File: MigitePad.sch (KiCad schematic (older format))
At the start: 74 parts, among them J1 OLED, J2 LED-Lily58-cache, SW1 SW_Push, SW2 Rotary_Encoder_Switch, U1 ProMicro

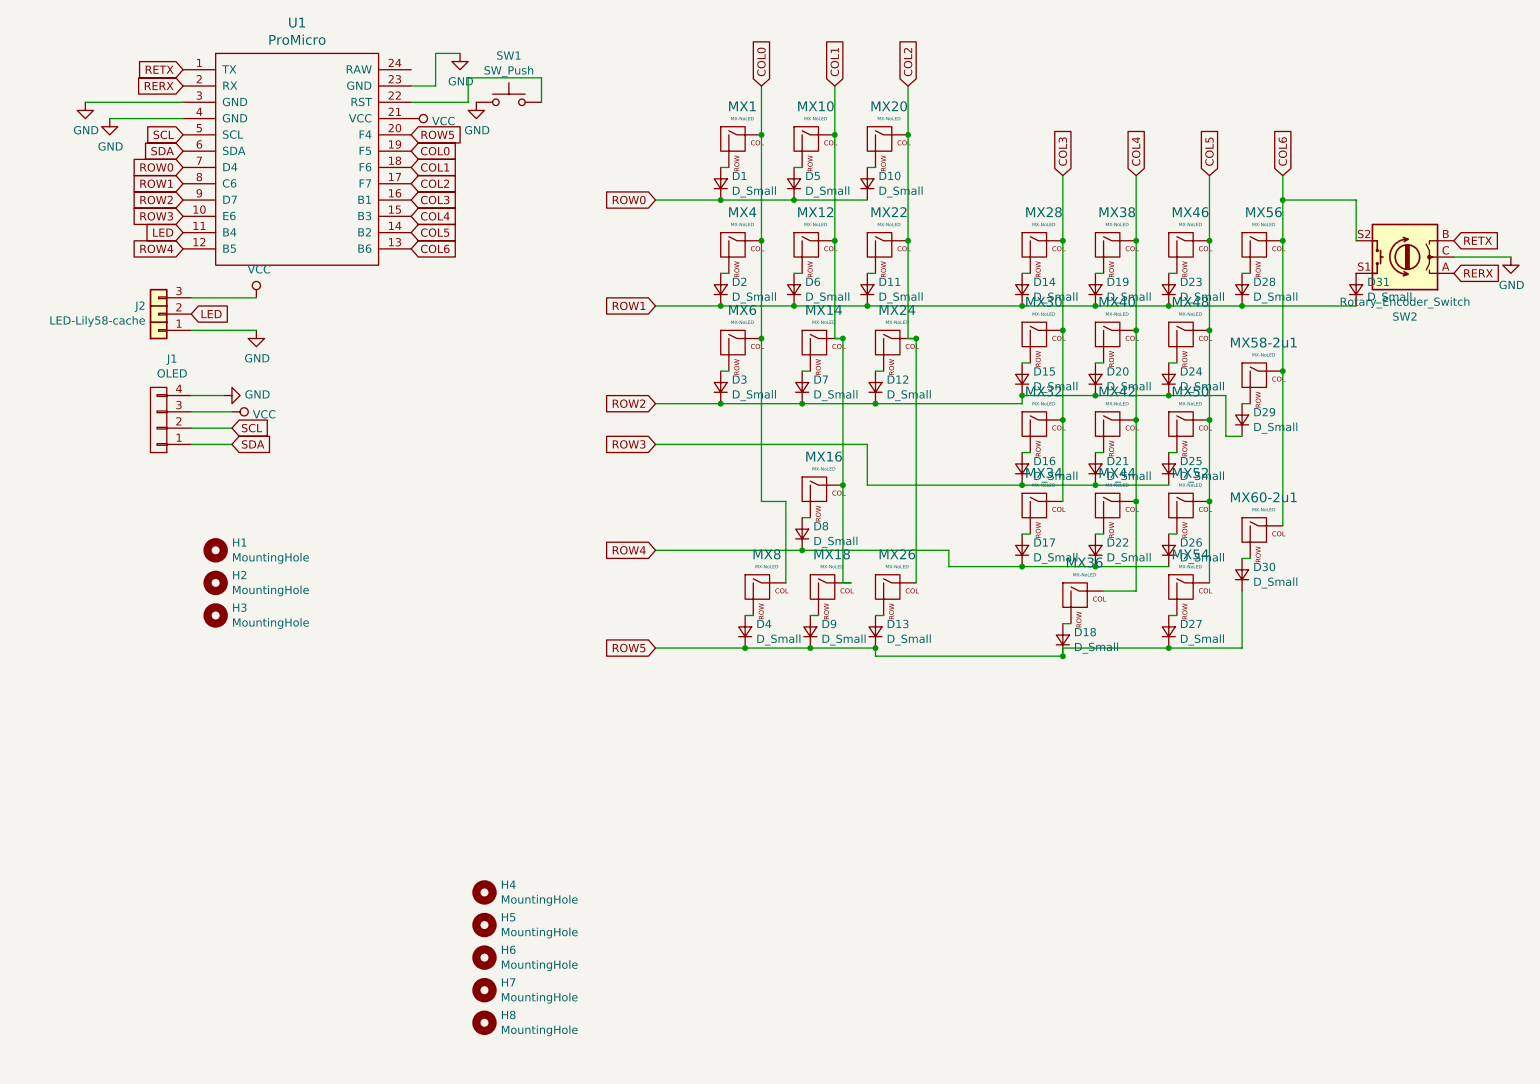
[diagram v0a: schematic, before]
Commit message: Rewired Encoder
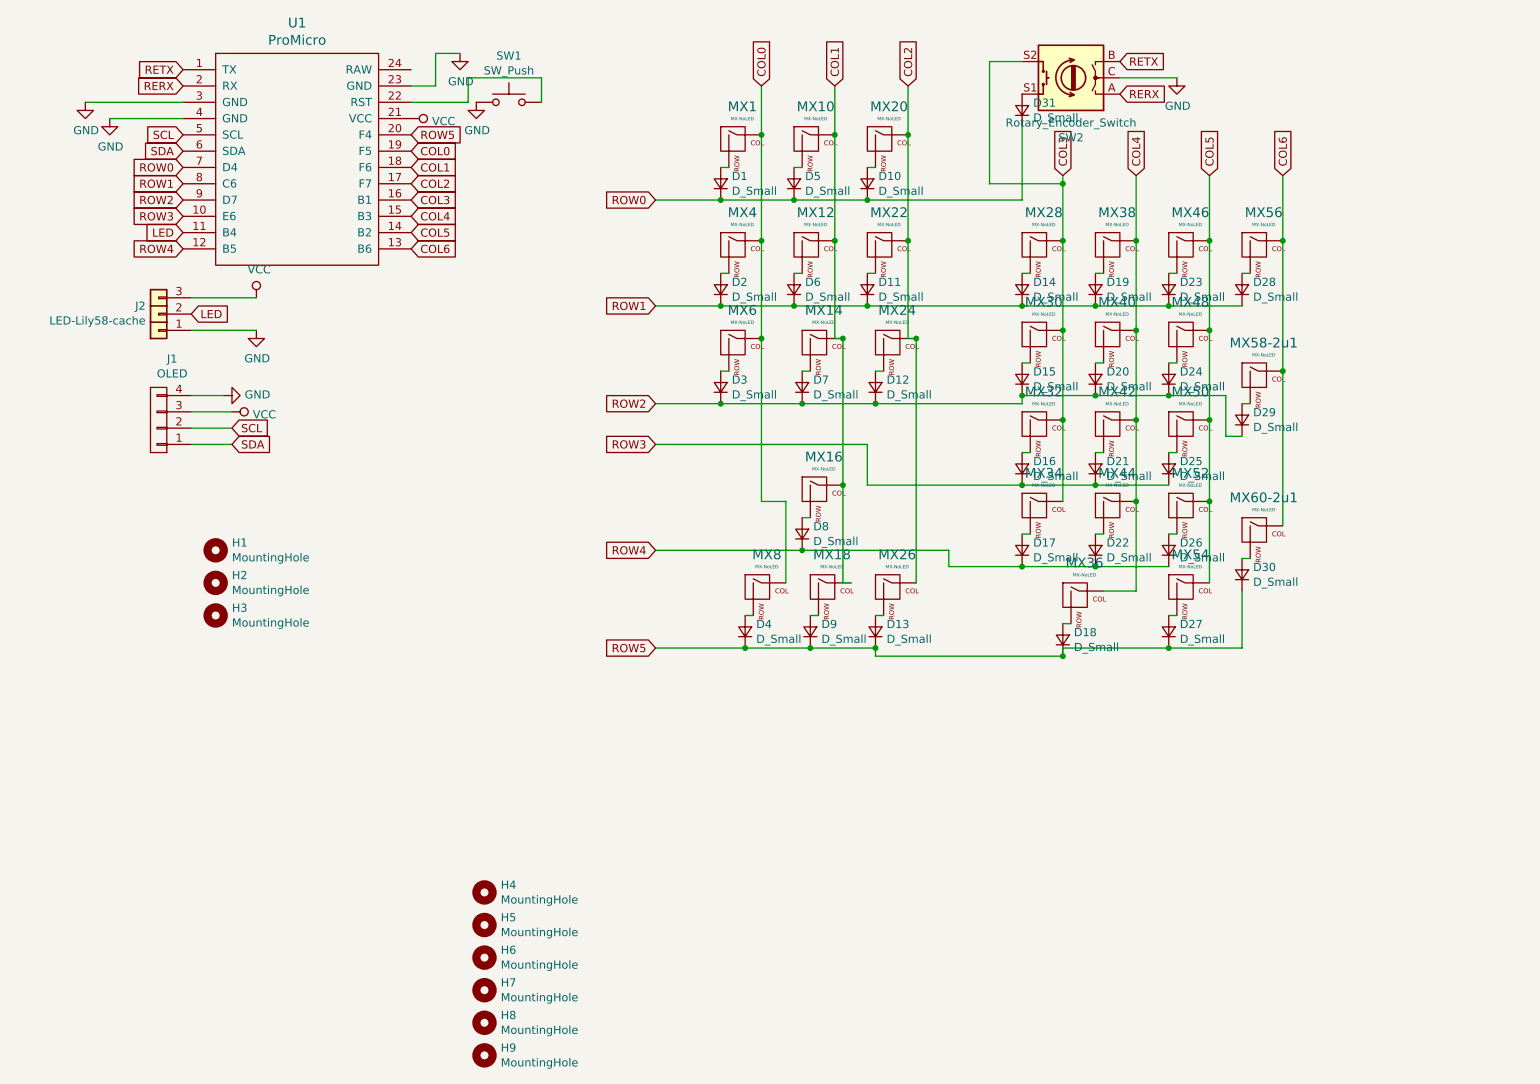
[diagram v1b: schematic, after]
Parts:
- added H9: MountingHole, Lily58-footprint:HOLE_M2_TH, symbol Mechanical:MountingHole
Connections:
- net COL3: now also SW2.S2
- net COL6: no longer SW2.S2
- net ROW0: now also D31.1 (K)
- net ROW1: no longer D31.1 (K)
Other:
- moved on the sheet: D31, SW2
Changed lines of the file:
@@
 	8250 2800 8250 3750
 Wire Wire Line
-	6900 2000 6900 1600
+	6900 2000 6900 1650
 Wire Wire Line
 	7350 2000 7350 1600
 Wire Wire Line
 	7800 2000 7800 1600
-Wire Wire Line
-	8250 2000 8250 1750
 Wire Wire Line
 	5700 2400 6650 2400
@@
 L Device:Rotary_Encoder_Switch SW2
 U 1 1 5E65AE52
-P 9000 2100
-F 0 "SW2" H 9000 2467 50  0000 C CNN
-F 1 "Rotary_Encoder_Switch" H 9000 2376 50  0000 C CNN
-F 2 "Keebio-Parts:RotaryEncoder_EC11" H 8850 2260 50  0001 C CNN
-F 3 "~" H 9000 2360 50  0001 C CNN
-	1    9000 2100
+P 6950 1000
+F 0 "SW2" H 6950 1367 50  0000 C CNN
+F 1 "Rotary_Encoder_Switch" H 6950 1276 50  0000 C CNN
+F 2 "Keebio-Parts:RotaryEncoder_EC11" H 6800 1160 50  0001 C CNN
+F 3 "~" H 6950 1260 50  0001 C CNN
+	1    6950 1000
 	-1   0    0    1
 $EndComp
@@
 L Device:D_Small D31
 U 1 1 5E668E53
-P 8700 2300
-F 0 "D31" V 8746 2232 50  0000 R CNN
-F 1 "D_Small" V 8655 2232 50  0000 R CNN
-F 2 "Lily58-footprint:Diode_TH_SOD123" V 8700 2300 50  0001 C CNN
-F 3 "~" V 8700 2300 50  0001 C CNN
-	1    8700 2300
+P 6650 1200
+F 0 "D31" V 6696 1132 50  0000 R CNN
+F 1 "D_Small" V 6605 1132 50  0000 R CNN
+F 2 "Lily58-footprint:Diode_TH_SOD123" V 6650 1200 50  0001 C CNN
+F 3 "~" V 6650 1200 50  0001 C CNN
+	1    6650 1200
 	0    -1   -1   0
 $EndComp
-Wire Wire Line
-	8000 2400 8700 2400
-Connection ~ 8000 2400
-Wire Wire Line
-	8700 2000 8700 1750
-Wire Wire Line
-	8700 1750 8250 1750
-Connection ~ 8250 1750
-Wire Wire Line
-	8250 1750 8250 1600
 Text GLabel 1500 950  0    50   Input ~ 0
 RETX
 Text GLabel 1500 1050 0    50   Input ~ 0
 RERX
-Text GLabel 9300 2000 2    50   Input ~ 0
+Text GLabel 7250 900  2    50   Input ~ 0
 RETX
-Text GLabel 9300 2200 2    50   Input ~ 0
+Text GLabel 7250 1100 2    50   Input ~ 0
 RERX
 $Comp
 L power:GND #PWR0110
 U 1 1 5E68B0C4
-P 9650 2100
-F 0 "#PWR0110" H 9650 1850 50  0001 C CNN
-F 1 "GND" H 9655 1927 50  0000 C CNN
-F 2 "" H 9650 2100 50  0001 C CNN
-F 3 "" H 9650 2100 50  0001 C CNN
-	1    9650 2100
-	1    0    0    -1
-$EndComp
-Wire Wire Line
-	9300 2100 9650 2100
+P 7600 1000
+F 0 "#PWR0110" H 7600 750 50  0001 C CNN
+F 1 "GND" H 7605 827 50  0000 C CNN
+F 2 "" H 7600 1000 50  0001 C CNN
+F 3 "" H 7600 1000 50  0001 C CNN
+	1    7600 1000
+	1    0    0    -1
+$EndComp
+Wire Wire Line
+	7250 1000 7600 1000
+$Comp
+L Mechanical:MountingHole H9
+U 1 1 5E65D16B
+P 3350 7000
+F 0 "H9" H 3450 7046 50  0000 L CNN
+F 1 "MountingHole" H 3450 6955 50  0000 L CNN
+F 2 "Lily58-footprint:HOLE_M2_TH" H 3350 7000 50  0001 C CNN
+F 3 "~" H 3350 7000 50  0001 C CNN
+	1    3350 7000
+	1    0    0    -1
+$EndComp
+Wire Wire Line
+	8250 1600 8250 2000
+Wire Wire Line
+	5700 1750 6650 1750
+Wire Wire Line
+	6650 1750 6650 1300
+Connection ~ 5700 1750
+Wire Wire Line
+	6650 900  6450 900
+Wire Wire Line
+	6450 900  6450 1650
+Wire Wire Line
+	6450 1650 6900 1650
+Connection ~ 6900 1650
+Wire Wire Line
+	6900 1650 6900 1600
 $EndSCHEMATC
